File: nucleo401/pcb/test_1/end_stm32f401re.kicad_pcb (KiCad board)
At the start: 2 copper layers, 24 parts, among them J2 USB_B_Micro, U2 NUCLEO-64

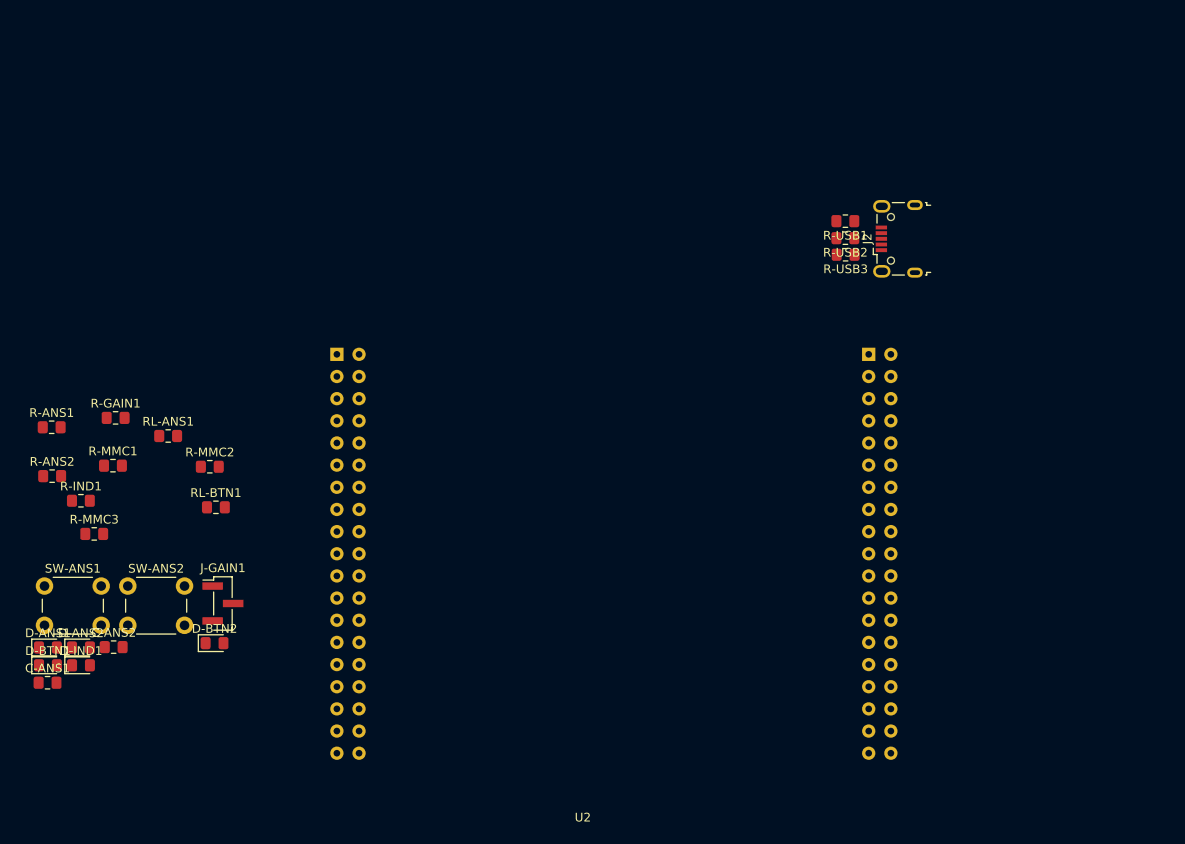
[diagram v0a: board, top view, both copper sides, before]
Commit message: PCB next proto design
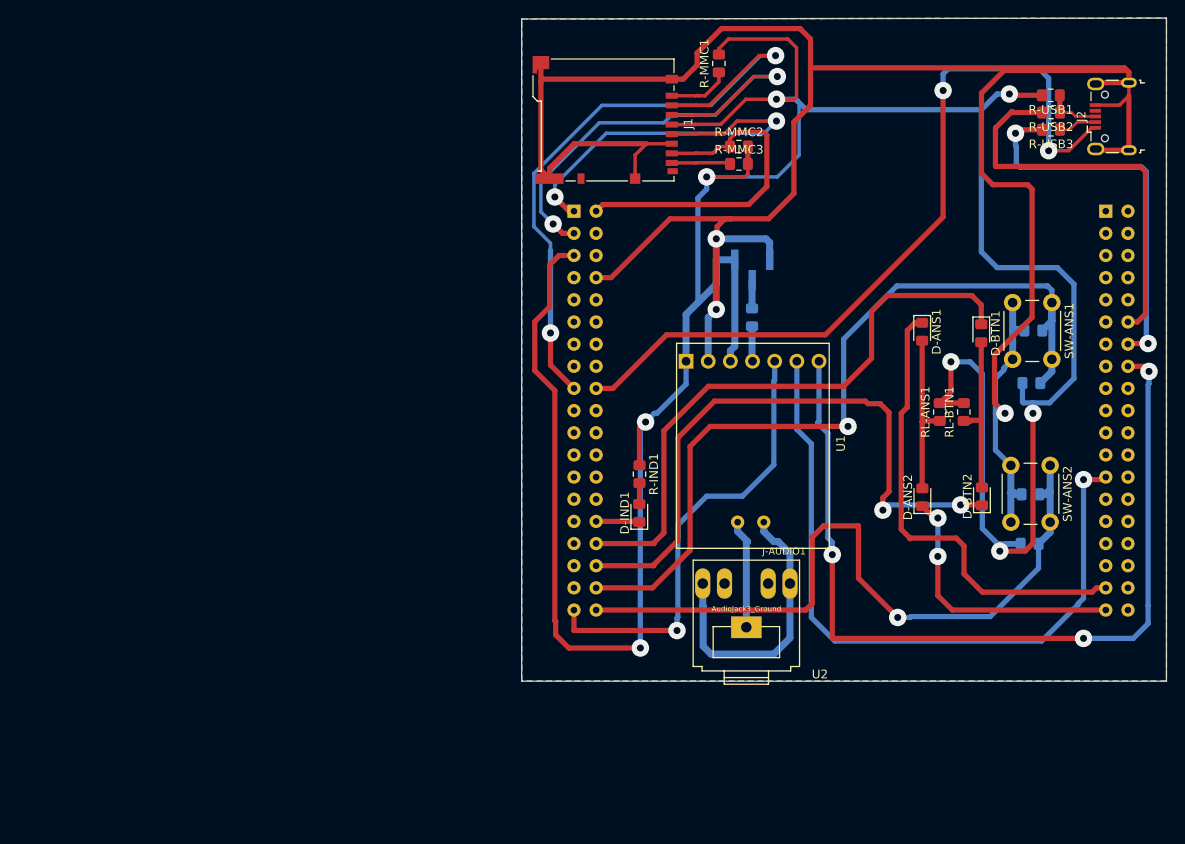
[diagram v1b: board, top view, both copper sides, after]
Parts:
- added J-AUDIO1: AudioJack3_Ground, user:Tayda_3.5mm_stereo_TRS_jack_A-853, F.Cu at (130.2, 132.4)
- added J1: Micro_SD_Card_Det, Connector_Card:microSD_HC_Hirose_DM3BT-DSF-PEJS, F.Cu at (114.0, 75.9)
- added U1: MAX98357_DAC, dacmax98:dacmax98357, F.Cu at (130.7, 113.0)
- C-ANS1, C-ANS2, J-GAIN1, R-ANS1, R-ANS2, R-GAIN1: moved to B.Cu
- moved C-ANS1 120.0 mm to (163.0, 100.0)
- moved SW-ANS1 120.0 mm to (165.2, 96.8), turned to 270 degrees
- moved D-BTN1 113.5 mm to (157.1, 100.3), turned to 270 degrees
- moved R-ANS1 112.4 mm to (162.8, 106.0)
- moved R-ANS2 112.3 mm to (162.6, 124.5)
- moved SW-ANS2 106.6 mm to (165.0, 115.5), turned to 270 degrees
- moved D-ANS1 106.5 mm to (150.3, 100.2), turned to 270 degrees
- moved C-ANS2 106.5 mm to (162.7, 118.8)
- moved D-ANS2 98.0 mm to (150.3, 119.1), turned to 90 degrees
- moved D-BTN2 89.5 mm to (157.2, 119.0), turned to 90 degrees
- moved RL-ANS1 88.5 mm to (152.3, 109.3), turned to 90 degrees
- moved RL-BTN1 86.4 mm to (155.1, 109.3), turned to 90 degrees
- moved R-MMC3 85.2 mm to (129.3, 80.9)
- moved R-MMC1 83.4 mm to (127.0, 69.4), turned to 90 degrees
- moved R-GAIN1 73.9 mm to (130.8, 98.5), turned to 90 degrees
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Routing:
- net VDD: track 0.00 -> 335.6 mm, vias 0 -> 8
- net GND: track 0.00 -> 290.3 mm, vias 0 -> 3
- net /DAC_LRC: track 0.00 -> 101.0 mm, vias 0 -> 3
- net /BTN_A: track 0.00 -> 95.2 mm, vias 0 -> 1
- net VCC: track 0.00 -> 91.9 mm, vias 0 -> 2
- net /BTN_B: track 0.00 -> 83.0 mm, vias 0 -> 1
- net /DAC_BCLK: track 0.00 -> 80.7 mm, vias 0 -> 1
- net /MMC_NSS: track 0.00 -> 74.1 mm, vias 0 -> 2
- net /LED_B: track 0.00 -> 72.0 mm, vias 0 -> 2
- net /LED_A: track 0.00 -> 68.7 mm
- net /MMC_MOSI: track 0.00 -> 54.3 mm, vias 0 -> 2
- net /LED_TRUE: track 0.00 -> 53.8 mm
- net /DAC_DIN: track 0.00 -> 52.1 mm, vias 0 -> 1
- net /USB_DP: track 0.00 -> 46.7 mm
- net /MMC_SCK: track 0.00 -> 45.3 mm, vias 0 -> 2
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- added copper zone on B.Cu, net (none)
- added copper zone on F.Cu, net (none)
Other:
- board outline added: 73.9 x 76 mm
- net class Default: clearance 0.2 -> 0.15; via_dia 0.8 -> 2; via_drill 0.4 -> 0.8
- rule trace_clearance: 0.2 -> 0.15
